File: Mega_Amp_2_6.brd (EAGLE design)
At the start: 36 x 41.9 mm, 77 parts, among them Q1 2SC945SOT23, Q2 2SC945SOT23

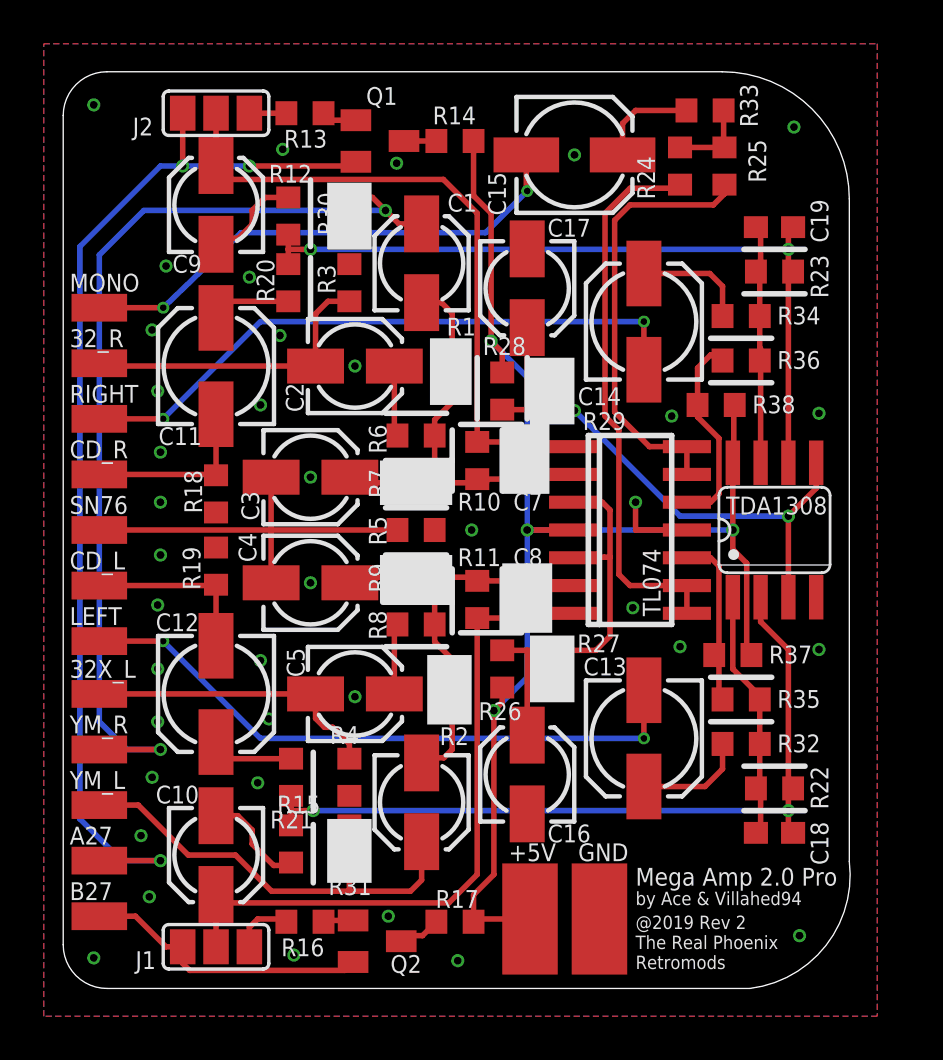
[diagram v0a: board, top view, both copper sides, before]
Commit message: Add files via upload
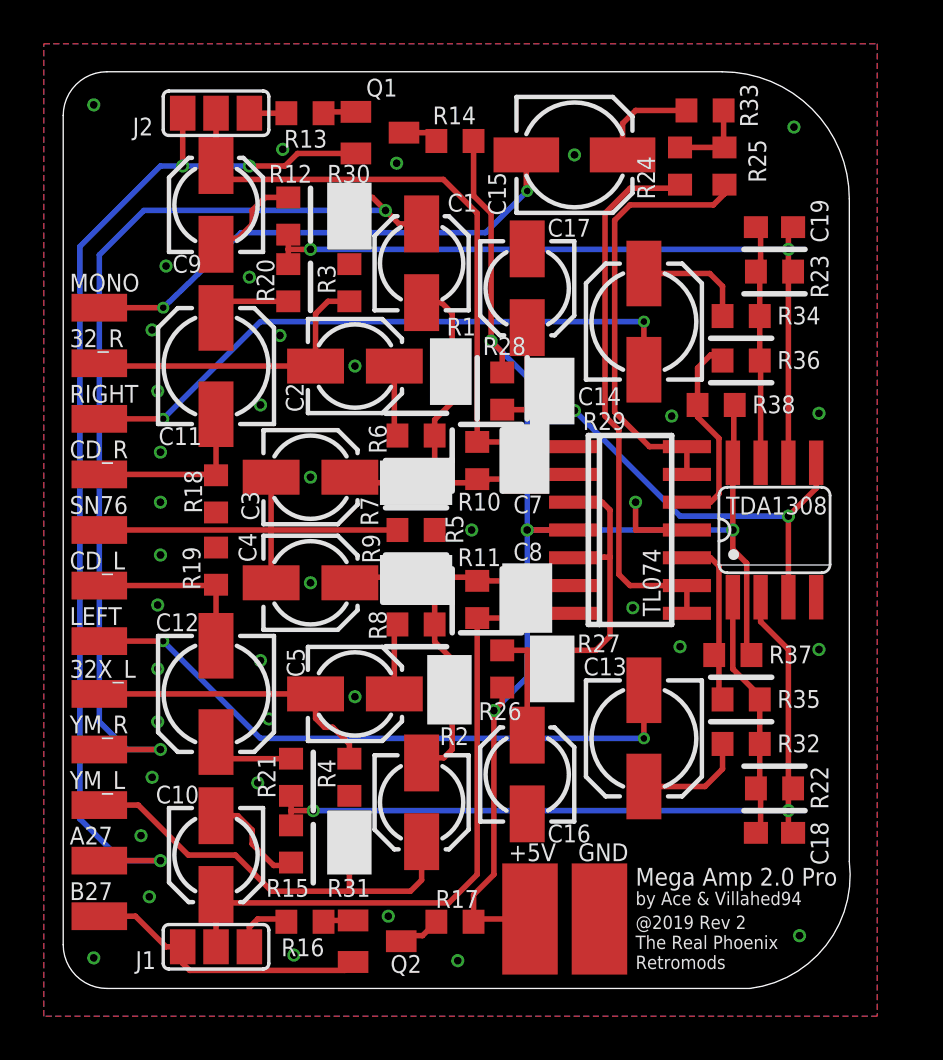
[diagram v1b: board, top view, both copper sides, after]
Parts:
- moved Q1 0.38 mm to (21.7, 41.7)
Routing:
- net N$42: track 11.9 -> 11.4 mm
